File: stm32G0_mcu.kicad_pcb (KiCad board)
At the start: 4 copper layers, 70 x 45 mm, 44 parts, among them J1 Conn_01x04_Pin, J2 Conn_01x06_Pin, J3 Conn_01x04_Pin, SW1 SW_Nidec_CAS-120A1, SW2 SW_Push, U1 STM32G0B0KETx, U7 FT230XS

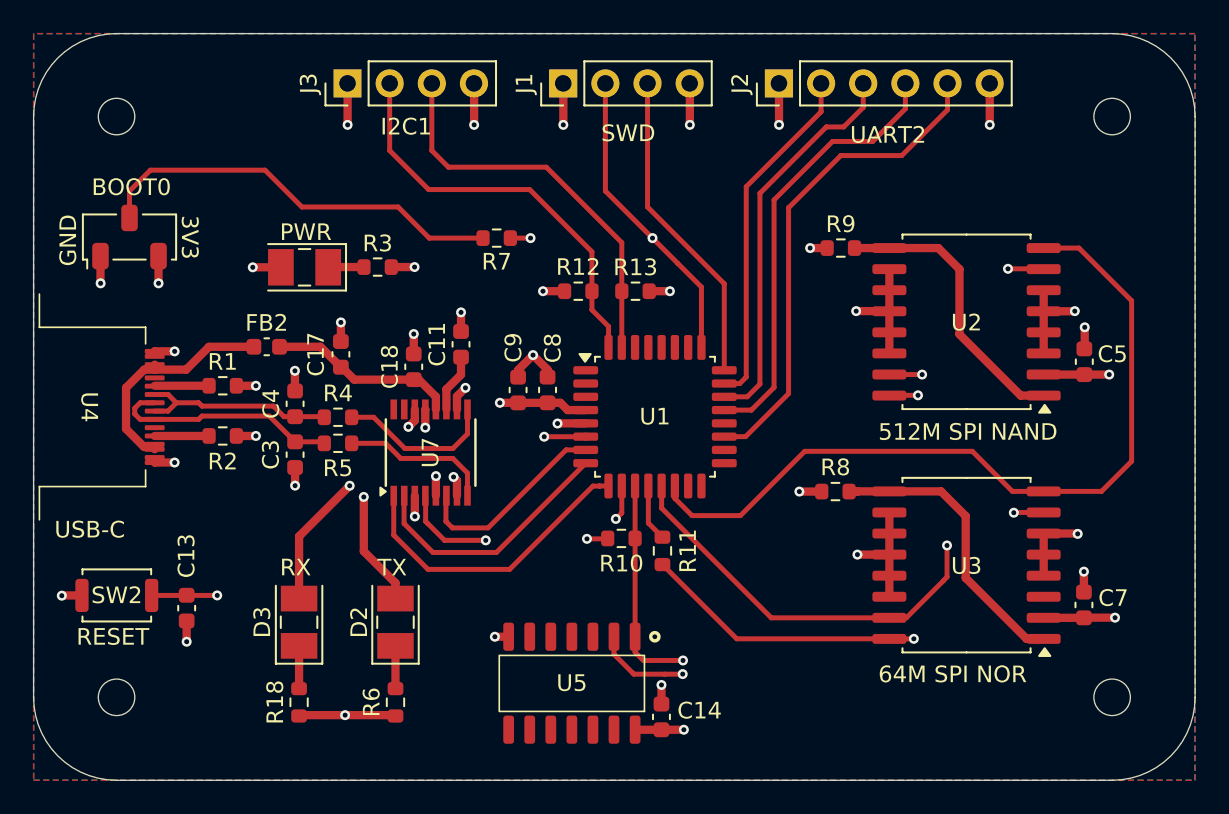
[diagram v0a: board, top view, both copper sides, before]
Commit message: adsad
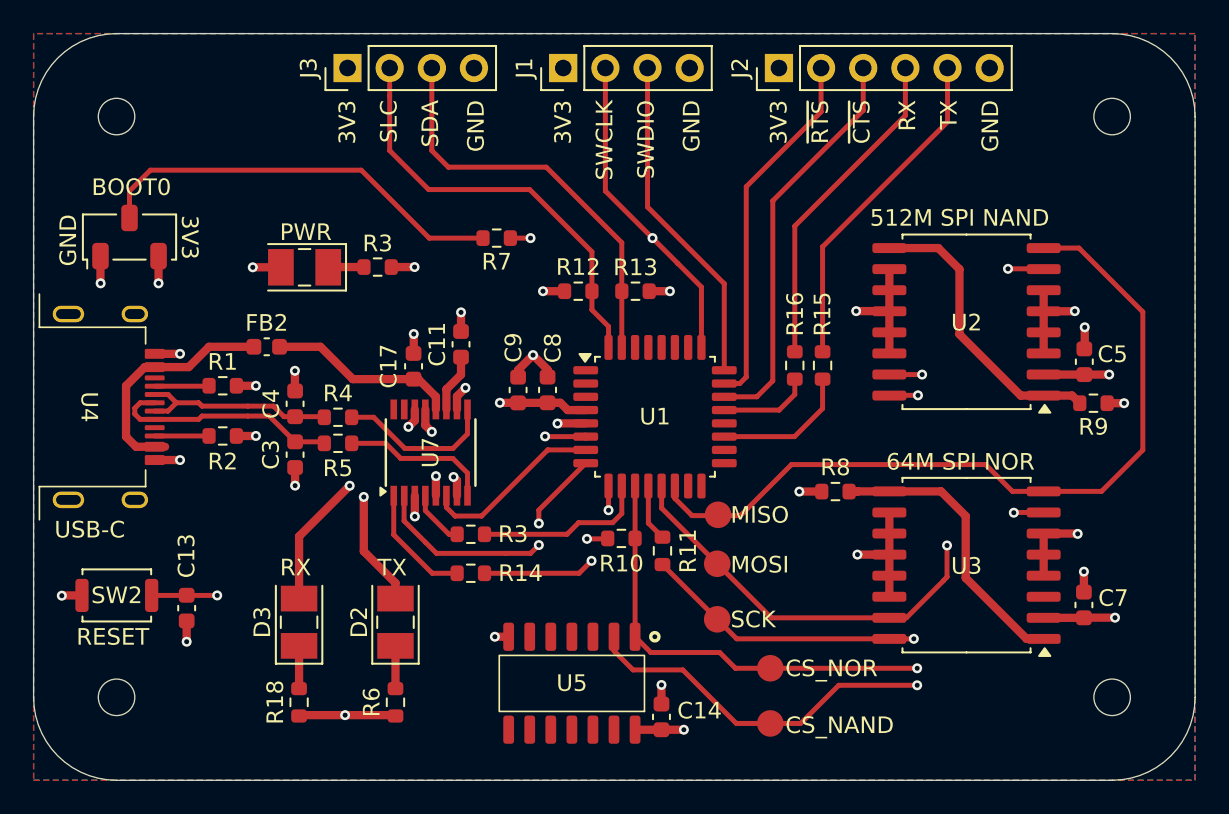
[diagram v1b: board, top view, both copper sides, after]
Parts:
- removed C18: 4u7, Capacitor_SMD:C_0603_1608Metric
- added R14: 120, Resistor_SMD:R_0603_1608Metric, F.Cu at (126.3, 112.5)
- added R15: 120, Resistor_SMD:R_0603_1608Metric, F.Cu at (147.6, 100.0)
- added R16: 120, Resistor_SMD:R_0603_1608Metric, F.Cu at (145.9, 100.0)
- added R3: 120, Resistor_SMD:R_0603_1608Metric, F.Cu at (126.3, 110.2)
- C11: value 47p -> 100n
- FB2: value FerriteBead -> 10u
- R12, R13: value 5k1 -> 1k8
- moved R9 17.9 mm to (163.9, 102.3), turned to 180 degrees
- moved C17 4.44 mm to (122.9, 100.0)
- moved J1 0.92 mm to (131.9, 82.1)
- moved J2 0.92 mm to (144.9, 82.1)
- moved J3 0.92 mm to (118.9, 82.1)
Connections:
- D2 pad 2: +3.3V -> Net-(D2-A)
- D3 pad 2: +3.3V -> Net-(D3-A)
- R1 pad 1: /POWER_SUPPLY/CC -> CC1
- R18 pad 2: +3.3V -> Net-(D3-A)
- R2 pad 1: /POWER_SUPPLY/CC -> CC2
- R6 pad 2: +3.3V -> Net-(D2-A)
- U4 pad : (no net) -> GND
- U4 pad A5: /POWER_SUPPLY/CC -> CC1
- U4 pad B5: /POWER_SUPPLY/CC -> CC2
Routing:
- net +3.3V: track 46.9 -> 34.3 mm, vias 17 -> 14
- net GND: track 60.5 -> 53.5 mm, vias 28 -> 24
- net /POWER_SUPPLY/CC: track 6.55 -> 0.00 mm
- net CC1: track 0.00 -> 3.29 mm
- net CC2: track 0.00 -> 3.28 mm
- net Net-(D3-A): track 0.00 -> 2.57 mm
- net Net-(D2-A): track 0.00 -> 2.57 mm
- net FLASH_NOR_CS: track 36.1 -> 38.4 mm
- net UART2_RX: track 16.2 -> 13.9 mm, vias 2 -> 0
- net ~{UART2_RTS}: track 15.6 -> 16.8 mm, vias 0 -> 2
- net UART1_RX: track 26.6 -> 25.4 mm
- net UART1_TX: track 29.8 -> 28.6 mm
- net ~{UART2_CTS}: track 12.1 -> 11.0 mm
- net ~{UART1_RTS}: track 21.1 -> 22.0 mm
- net SWDIO: track 19.2 -> 20.1 mm
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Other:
- board text added: "CS_NAND"
- board text added: "CS_NOR"
- board text added: "MISO"
- board text added: "MOSI"
- board text added: "SCK"
- board text added: "SDA"
- board text added: "SLC"
- board text added: "SWCLK"
- board text added: "SWDIO"
- board text added: "~{CTS}"
- board text added: "~{RTS}"
- board text removed: "I2C1"
- board text removed: "KabelitzJ STM32G0 Dev Board Rev. 1 29.10.2024"
- board text removed: "SWD"
- board text removed: "UART2"
